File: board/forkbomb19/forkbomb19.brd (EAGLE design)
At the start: 89.2 x 83.7 mm, 75 parts, among them T3 MMUN2133LT1G, U1 ESP-WROOM-03, U4 TPS61090RSAR

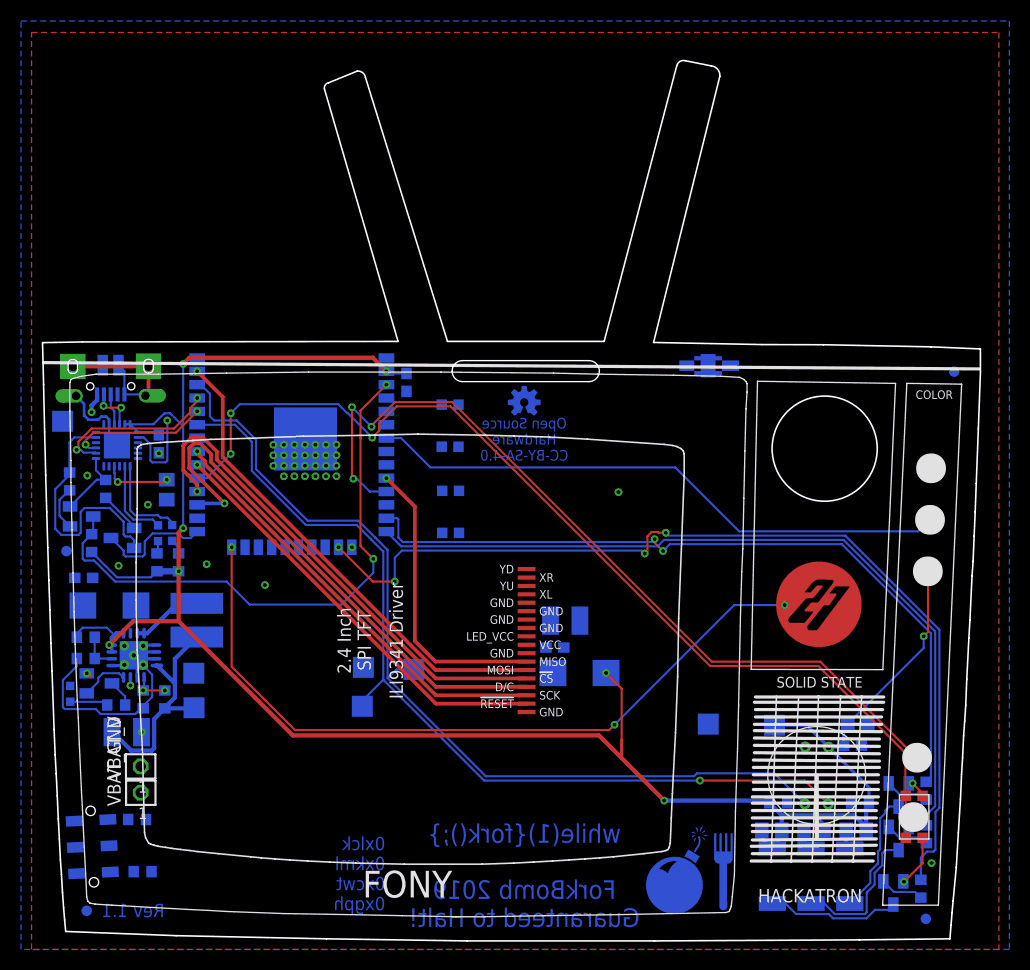
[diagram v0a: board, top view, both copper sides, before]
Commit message: finished rev 1.1
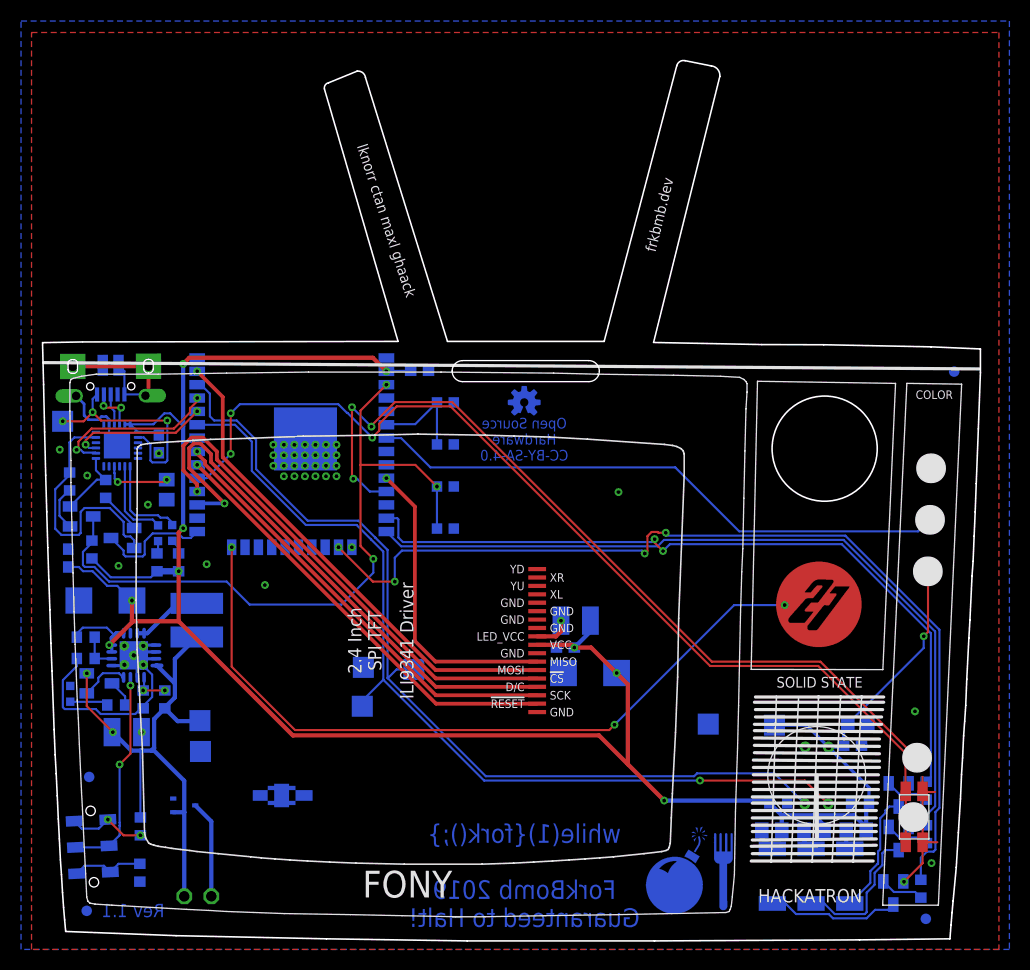
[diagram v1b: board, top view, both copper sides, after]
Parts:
- removed VBAT_GND, VBAT_V: POT_GND, con-samtec:TSW-101-XX-G-S
- added N1: MCH3484, forkbomb19:MCH3484
- added VBAT+, VBAT-: POT_GND, con-samtec:TSW-101-XX-G-S
- R24: value 1.33M -> 1.13M
- moved FID4 21.6 mm to (4.62, 15.4)
- moved TP_BATT_GND 7.47 mm to (15.2, 17.8)
- moved C5 2.40 mm to (2.63, 36.2), turned to 90 degrees
- moved C1 1.67 mm to (36.1, 54.0), turned to 180 degrees
- moved TP_BATT_VBAT 1.34 mm to (15.2, 20.7)
- moved C13 1.00 mm to (52.3, 25.3)
- moved C14 1.00 mm to (49.9, 27.7)
- moved R14 1.00 mm to (50.9, 30.2)
- moved U$2 1.00 mm to (47.2, 28.3)
- moved R18 0.73 mm to (9.50, 10.7), turned to 270 degrees
- moved HARDRST 0.65 mm to (38.5, 41.0)
- moved C4 0.61 mm to (6.17, 32.2), turned to 180 degrees
- moved R1 0.61 mm to (4.89, 37.0)
- moved SOFTRESET 0.50 mm to (38.5, 49.0)
- moved R9 0.28 mm to (9.44, 6.27), turned to 270 degrees
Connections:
- removed net I2C_GND: TP_I2C_GND.TP
- new net N$18: N1.D, VBAT-.1
- net GND: now also N1.S, TP_I2C_GND.TP; no longer VBAT_GND.1
- net VBAT: now also N1.G, VBAT+.1; no longer VBAT_V.1
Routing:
- net VBAT: track 23.8 -> 53.7 mm, vias 1 -> 2
- net ENABLE: track 1.09 -> 20.1 mm, vias 1 -> 2
- net +3V3: track 219.3 -> 236.5 mm, vias 8 -> 10
- net EN: track 54.6 -> 67.0 mm, vias 2 -> 3
- net VBUS: track 10.5 -> 21.1 mm, vias 2 -> 3
- net N$2: track 0.08 -> 9.69 mm
- net N$18: track 0.00 -> 9.27 mm
- net N$3: track 0.00 -> 7.57 mm, vias 0 -> 2
- net N$13: track 0.00 -> 6.89 mm
- net GND: track 61.1 -> 66.6 mm, vias 40 -> 41
- net N$1: track 0.00 -> 3.48 mm, vias 0 -> 1
- net SCRN_RST: track 40.7 -> 41.7 mm
- net SCRN_MOSI: track 46.5 -> 47.5 mm
- net SCRN_MISO: track 28.0 -> 29.0 mm
- net SCRN_D/CX: track 51.6 -> 52.6 mm
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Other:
- board text added: "frkbmb.dev"
- board text added: "lknorr ctan maxl ghaack"
- board text removed: "0xlck 0xkml 0xcwt 0xgph"
